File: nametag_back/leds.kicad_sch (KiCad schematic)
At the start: 55 parts, among them Q1 BSS138

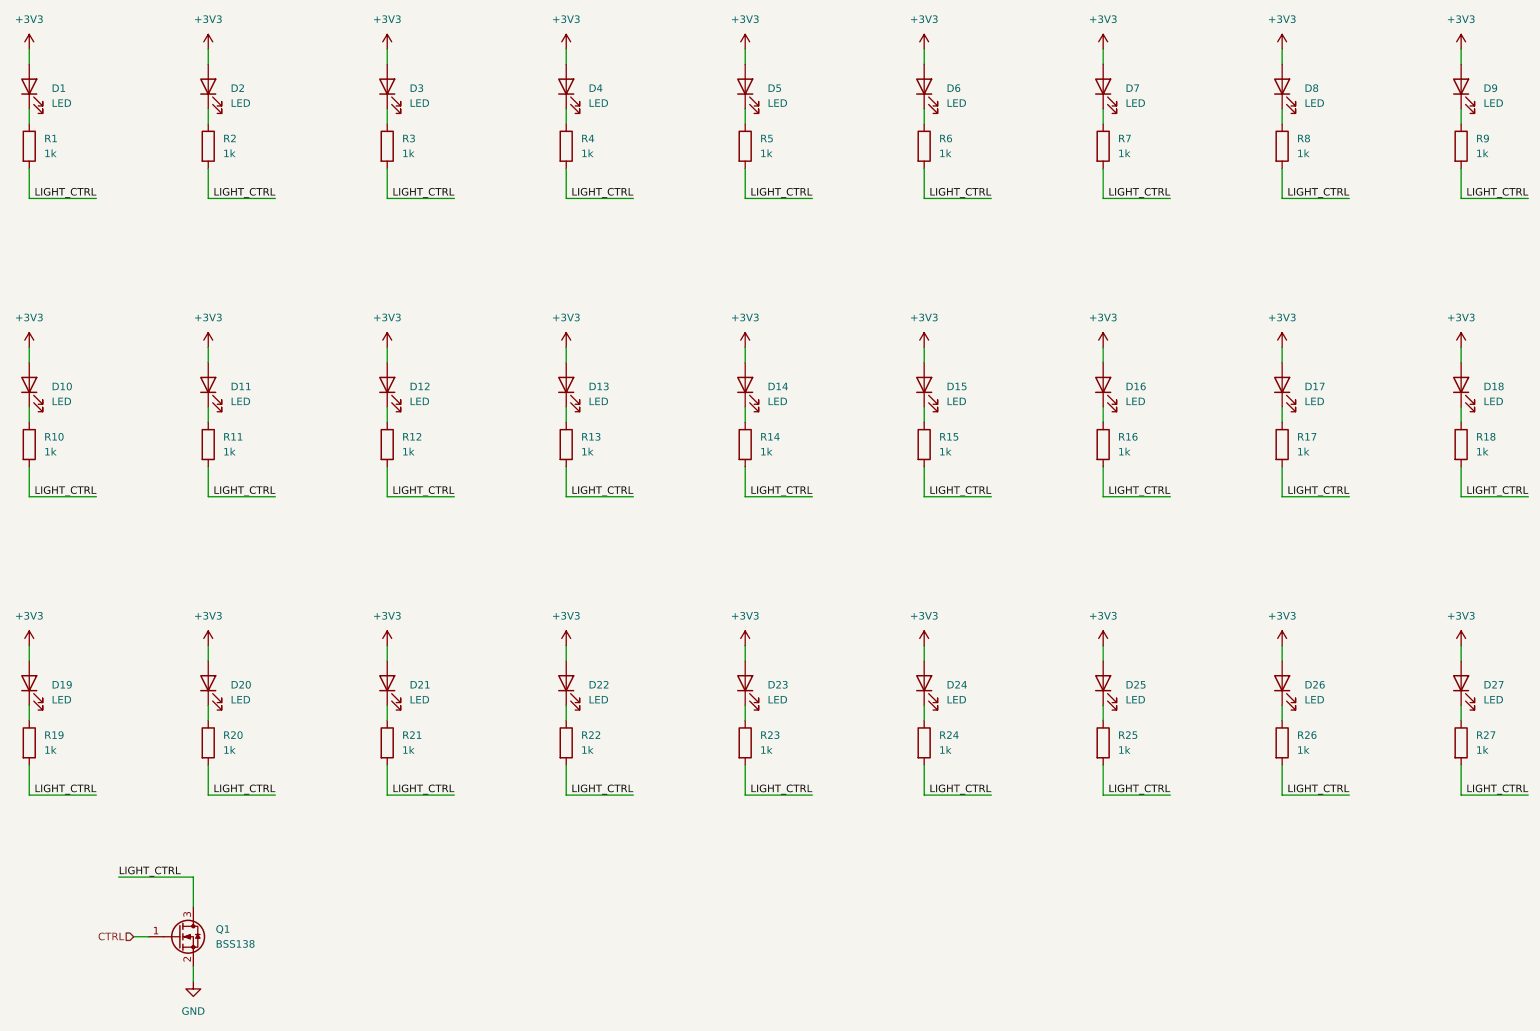
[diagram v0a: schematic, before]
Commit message: Push new fab files
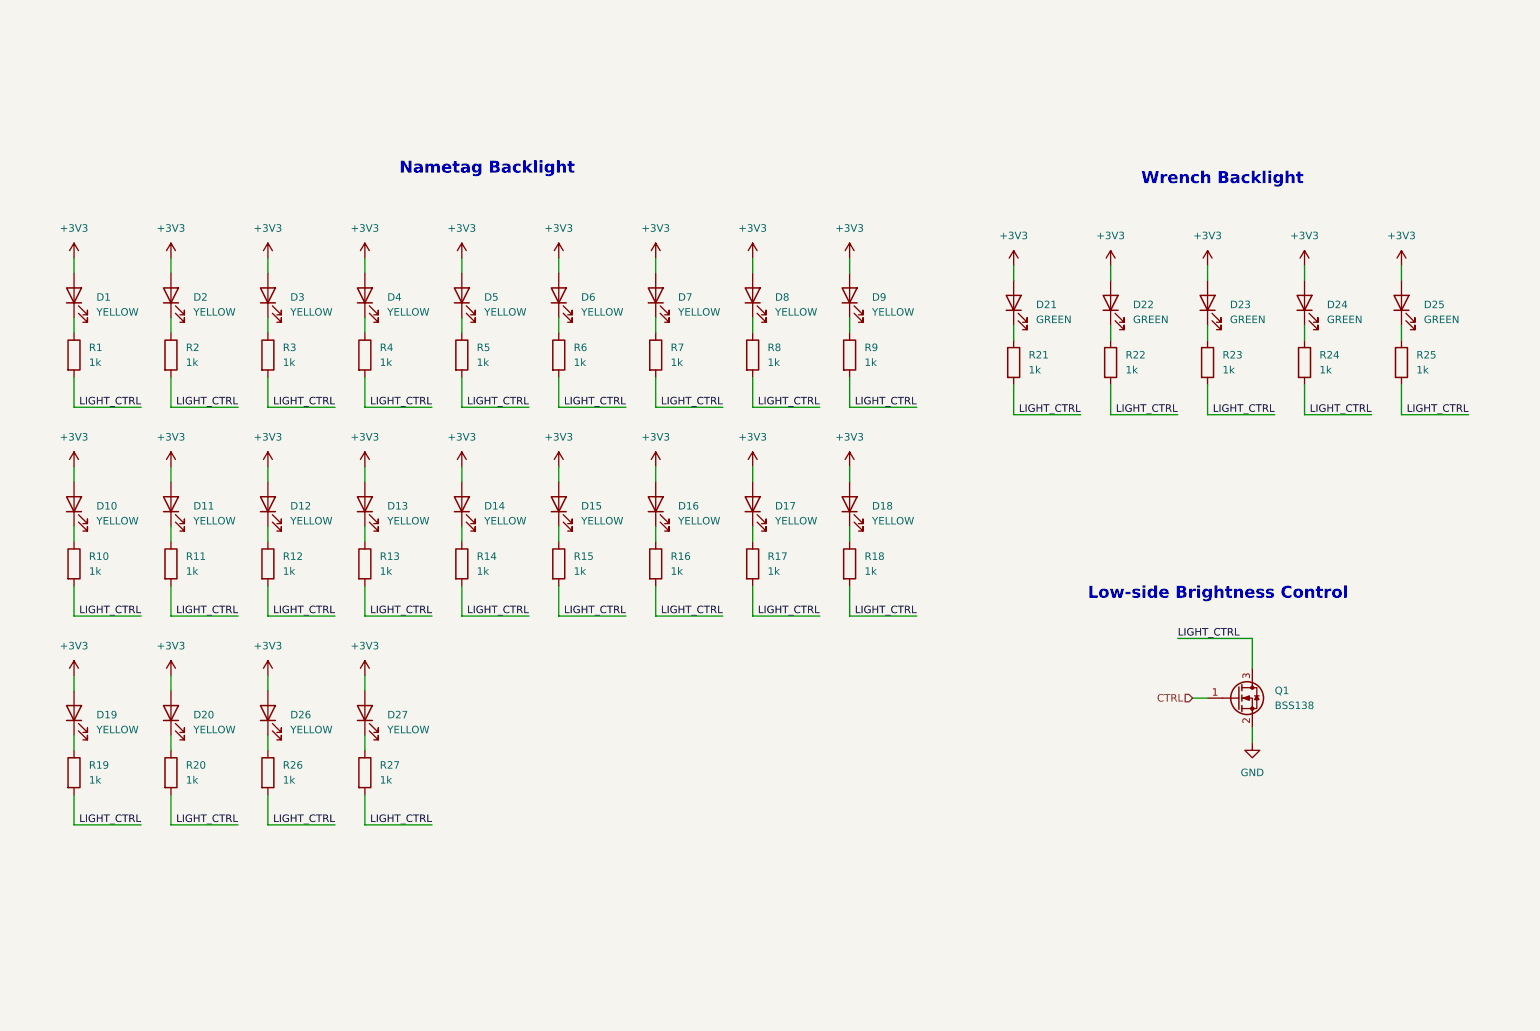
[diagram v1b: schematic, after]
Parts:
- D1, D10, D11, D12, D13, D14, D15, D16, D17, D18, D19, D2, D20, D26, D27, D3, D4, D5, D6, D7, D8, D9: value LED -> YELLOW
- D21, D22, D23, D24, D25: value LED -> GREEN
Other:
- note added: "Low-side Brightness Control"
- note added: "Nametag Backlight"
- note added: "Wrench Backlight"
- company: (none) -> Stan Okrasinski
- title: (none) -> Two-tier nametag - back
- moved on the sheet: D1, D10, D11, D12, D13, D14, D15, D16, D17, D18, D19, D2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
